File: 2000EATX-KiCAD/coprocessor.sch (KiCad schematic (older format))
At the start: 31 parts, among them CN600 Amiga-2000-CPU-Slot, U600 74LS245, U601 74LS245, U602 74LS245, U603 74LS245, U604 74LS245, U605 74LS245

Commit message: Add files via upload
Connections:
- wire segments 343 -> 338
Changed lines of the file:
@@
 $Descr A4 11693 8268
 encoding utf-8
-Sheet 4 9
+Sheet 4 10
 Title ""
 Date ""
@@
 	1500 1550 1500 1600
 $Comp
-L Amiga~3000~library:GND #PWR0123
+L power:GND #PWR0123
 U 1 1 604D2A89
 P 1500 6250
@@
 Connection ~ 2100 1750
 $Comp
-L Amiga~3000~library:+5V #PWR0124
+L power:+5V #PWR0124
 U 1 1 604D882A
 P 2100 1550
@@
 $EndComp
 $Comp
-L Amiga~3000~library:-5V #PWR0125
+L power:-5V #PWR0125
 U 1 1 604D8A9E
 P 2250 1350
@@
 $EndComp
 $Comp
-L Amiga~3000~library:+12V #PWR0126
+L power:+12V #PWR0126
 U 1 1 604DB1C1
 P 2400 1550
@@
 NoConn ~ 5300 1800
 $Comp
-L Amiga~3000~library:GND #PWR0127
+L power:GND #PWR0127
 U 1 1 60551069
 P 5800 2400
@@
 $EndComp
 $Comp
-L Amiga~3000~library:GND #PWR0128
+L power:GND #PWR0128
 U 1 1 6056F1B9
 P 6850 4150
@@
 $EndComp
 $Comp
-L Amiga~3000~library:GND #PWR0129
+L power:GND #PWR0129
 U 1 1 6056F9E8
 P 5850 5650
@@
 BD8
 $Comp
-L Amiga~3000~library:GND #PWR0130
+L power:GND #PWR0130
 U 1 1 605B732B
 P 10250 2800
@@
 $EndComp
 $Comp
-L Amiga~3000~library:GND #PWR0131
+L power:GND #PWR0131
 U 1 1 605B78D1
 P 10250 5050
@@
 	9750 4450 8800 4450
 $Comp
-L Amiga~3000~library:GND #PWR0132
+L power:GND #PWR0132
 U 1 1 607375B5
 P 7850 1800
@@
 $EndComp
 $Comp
-L Amiga~3000~library:GND #PWR0133
+L power:GND #PWR0133
 U 1 1 6073AFFD
 P 7900 4250
@@
 _BAS
 $Comp
-L Amiga~3000~library:GND #PWR0134
+L power:GND #PWR0134
 U 1 1 60B411F4
 P 3750 7500
@@
 $EndComp
 $Comp
-L Amiga~3000~library:+5V #PWR0135
+L power:+5V #PWR0135
 U 1 1 60B454E3
 P 4400 5650
 F 0 "#PWR0135" H 4400 5500 50  0001 C CNN
-F 1 "+5V" H 4417 5873 50  0000 C CNN
+F 1 "+5V" H 4400 5800 50  0000 C CNN
 F 2 "" H 4400 5650 50  0001 C CNN
 F 3 "" H 4400 5650 50  0001 C CNN
@@
 $EndComp
 $Comp
-L Amiga~3000~library:GND #PWR0136
+L power:GND #PWR0136
 U 1 1 60B78755
 P 3250 7200
@@
 $EndComp
 $Comp
-L Amiga~3000~library:+5V #PWR0137
+L power:+5V #PWR0137
 U 1 1 60E422B1
 P 3450 5800
@@
 $EndComp
 $Comp
-L Amiga~3000~library:GND #PWR0138
+L power:GND #PWR0138
 U 1 1 60E42986
 P 3150 5800
@@
 Wire Wire Line
 	3450 5900 3750 5900
-Connection ~ 3450 5800
 $Comp
 L Device:C_Small C602
@@
 $EndComp
 $Comp
-L Amiga~3000~library:GND #PWR0139
+L power:GND #PWR0139
 U 1 1 60E7B497
 P 10900 3450
@@
 $EndComp
 $Comp
-L Amiga~3000~library:GND #PWR0140
+L power:GND #PWR0140
 U 1 1 60E7BCF4
 P 10800 1200
@@
 $EndComp
 $Comp
-L Amiga~3000~library:GND #PWR0141
+L power:GND #PWR0141
 U 1 1 60E7CCB0
 P 6350 800
@@
 $EndComp
 $Comp
-L Amiga~3000~library:GND #PWR0142
+L power:GND #PWR0142
 U 1 1 60E7E9FD
 P 7500 2400
@@
 $EndComp
 $Comp
-L Amiga~3000~library:+5V #PWR0143
+L power:+5V #PWR0143
 U 1 1 60E89AA3
 P 6150 4150
@@
 	4200 850  4200 3750
 $Comp
-L Amiga~3000~library:+5V #PWR0144
+L power:+5V #PWR0144
 U 1 1 60FCDD63
 P 7150 2400
@@
 	1    0    0    -1
 $EndComp
-Wire Wire Line
-	7300 2400 7150 2400
-Connection ~ 7150 2400
-Wire Wire Line
-	7150 2400 6850 2400
-$Comp
-L Amiga~3000~library:+5V #PWR0145
+$Comp
+L power:+5V #PWR0145
 U 1 1 60FE91B2
 P 6050 800
@@
 $EndComp
 $Comp
-L Amiga~3000~library:+5V #PWR0146
+L power:+5V #PWR0146
 U 1 1 60FE967D
 P 10500 1200
@@
 $EndComp
 $Comp
-L Amiga~3000~library:+5V #PWR0147
+L power:+5V #PWR0147
 U 1 1 60FE9CDB
 P 10500 3450
@@
 	1    0    0    -1
 $EndComp
-Wire Wire Line
-	10250 3450 10500 3450
-Connection ~ 10500 3450
-Wire Wire Line
-	10500 3450 10700 3450
-Wire Wire Line
-	10600 1200 10500 1200
-Connection ~ 10500 1200
-Wire Wire Line
-	10500 1200 10250 1200
-Wire Wire Line
-	5800 800  6050 800
-Connection ~ 6050 800
-Wire Wire Line
-	6050 800  6150 800
-$Comp
-L Amiga~3000~library:GND #PWR0148
+$Comp
+L power:GND #PWR0148
 U 1 1 610452A3
 P 5300 2100
@@
 $EndComp
 $Comp
-L Amiga~3000~library:GND #PWR0149
+L power:GND #PWR0149
 U 1 1 61045A56
 P 5350 5350
@@
 $EndComp
 $Comp
-L Amiga~3000~library:GND #PWR0150
+L power:GND #PWR0150
 U 1 1 610463ED
 P 6350 3700
@@
 Wire Wire Line
 	6850 4150 6850 4000
-Connection ~ 6850 4150
-Wire Wire Line
-	6500 4150 6150 4150
 Wire Wire Line
 	5850 4050 6000 4050
 Wire Wire Line
 	6000 4050 6000 4150
-Wire Wire Line
-	6000 4150 6150 4150
-Connection ~ 6150 4150
 Text GLabel 7450 4950 0    47   Input ~ 0
 _DBOE
@@
 Wire Wire Line
 	3100 1700 3100 2550
+Wire Wire Line
+	6850 2400 7300 2400
+Wire Wire Line
+	10250 3450 10700 3450
+Wire Wire Line
+	10250 1200 10600 1200
+Wire Wire Line
+	5800 800  6150 800
+Wire Wire Line
+	6000 4150 6500 4150
 $EndSCHEMATC

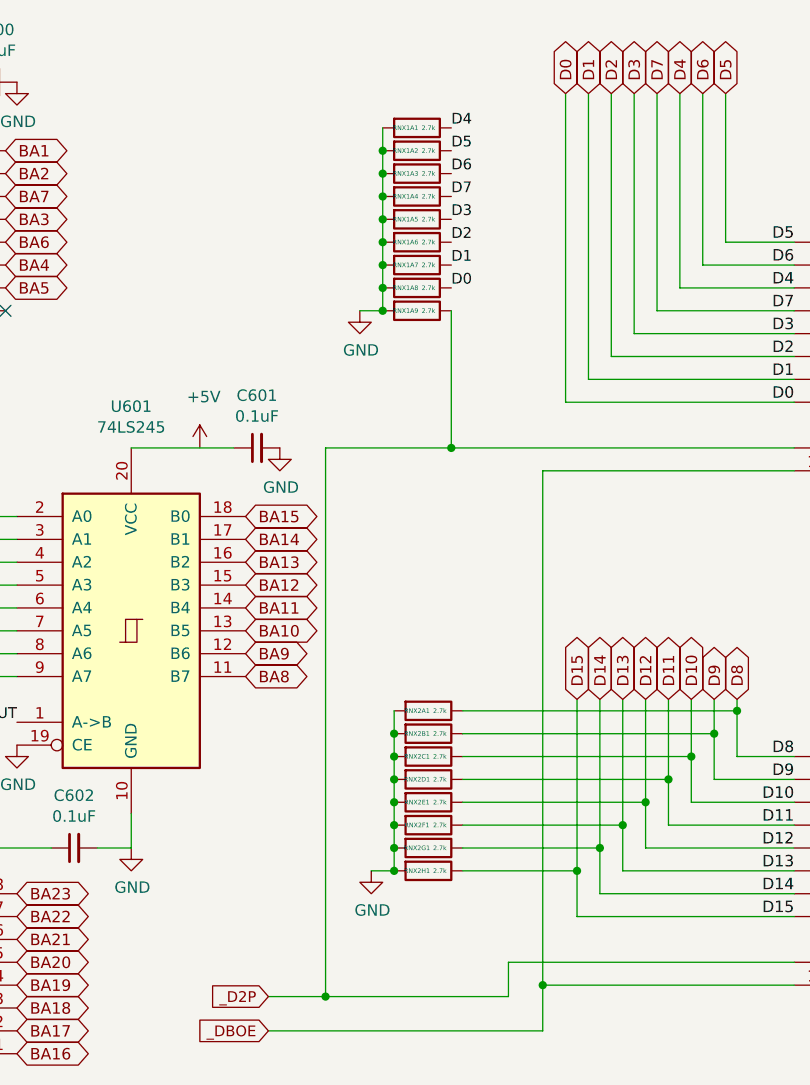
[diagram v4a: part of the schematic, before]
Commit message: Add files via upload
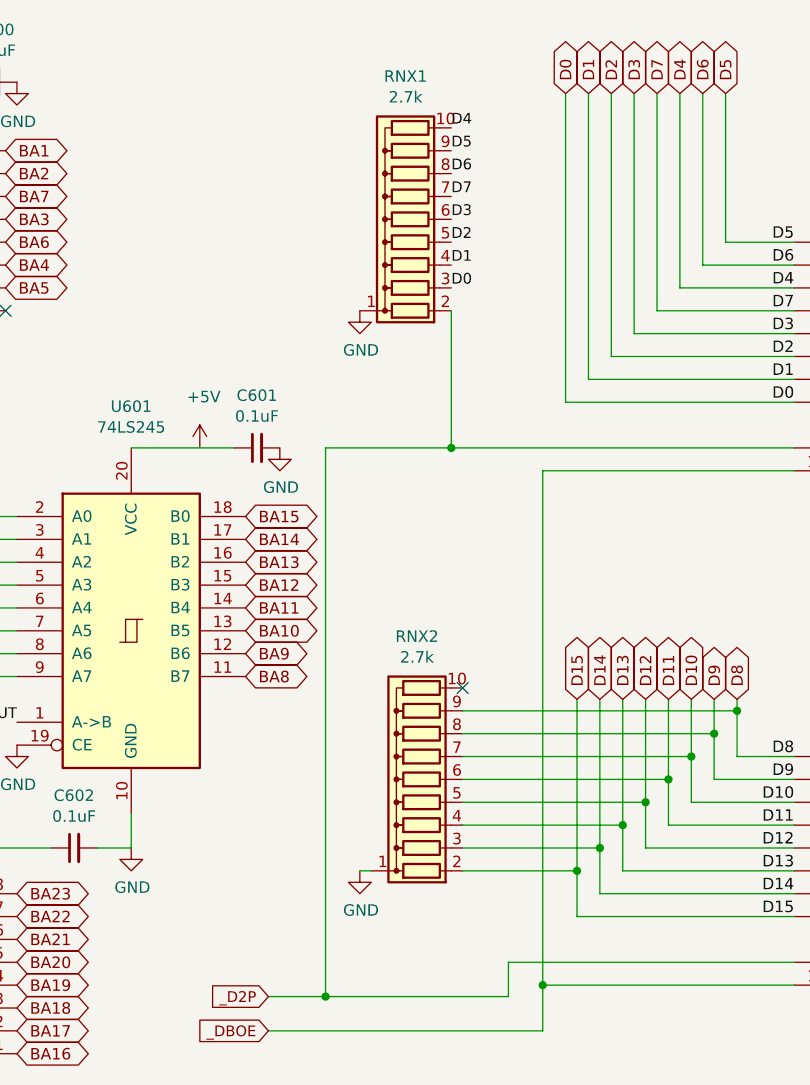
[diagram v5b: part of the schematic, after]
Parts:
- removed RNX1A1, RNX1A2, RNX1A3, RNX1A4, RNX1A5, RNX1A6, RNX1A7, RNX1A8, RNX1A9, RNX2A1, RNX2B1, RNX2C1, RNX2D1, RNX2E1, RNX2F1, RNX2G1, RNX2H1: 2.7k, Resistor_SMD:R_1206_3216Metric, symbol Device:R
- added RNX1, RNX2: 2.7k, Resistor_THT:R_Array_SIP10, symbol Device:R_Network09
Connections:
- net D0: now also RNX1.3 (R2)
- net D1: now also RNX1.4 (R3)
- net D10: now also RNX2.7 (R6)
- net D11: now also RNX2.6 (R5)
- net D12: now also RNX2.5 (R4)
- net D13: now also RNX2.4 (R3)
- net D14: now also RNX2.3 (R2)
- net D15: now also RNX2.2 (R1)
- net D2: now also RNX1.5 (R4)
- net D3: now also RNX1.6 (R5)
- net D4: now also RNX1.10 (R9)
- net D5: now also RNX1.9 (R8)
- net D6: now also RNX1.8 (R7)
- net D7: now also RNX1.7 (R6)
- net D8: now also RNX2.9 (R8)
- net D9: now also RNX2.8 (R7)
- net GND: now also RNX1.1 (common), RNX2.1 (common)
- net _D2P: now also RNX1.2 (R1)
- no-connect marks 2 -> 3

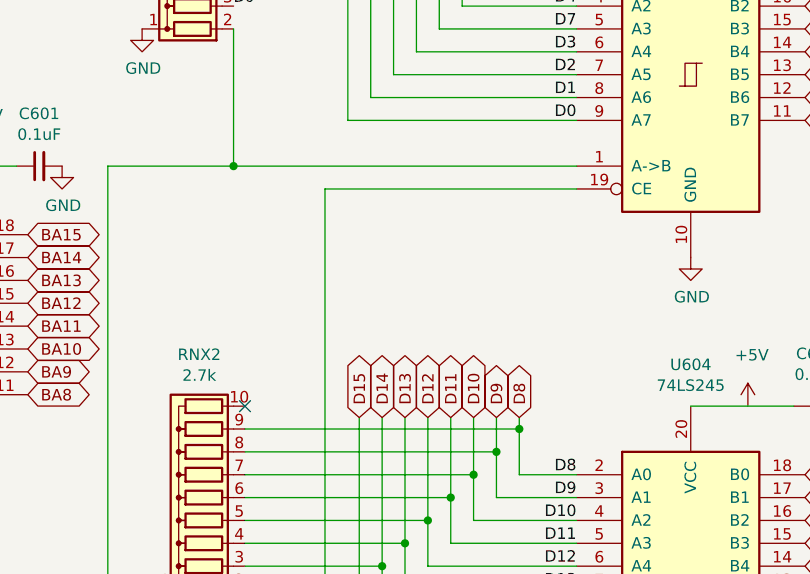
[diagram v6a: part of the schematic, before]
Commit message: Add files via upload
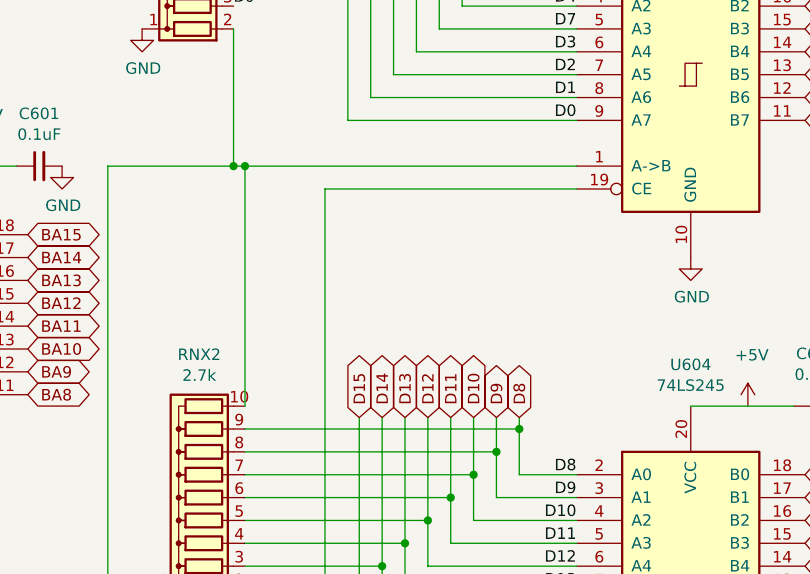
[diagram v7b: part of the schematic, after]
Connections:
- net _D2P: now also RNX2.10 (R9)
- no-connect marks 3 -> 2
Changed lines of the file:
@@
 Connection ~ 8250 2400
 Wire Wire Line
-	8250 2400 9750 2400
+	8250 2400 8300 2400
 Wire Wire Line
 	7450 4950 8650 4950
@@
 Wire Wire Line
 	7850 4250 7900 4250
-NoConn ~ 8300 3450
+Wire Wire Line
+	8300 3450 8300 2400
+Connection ~ 8300 2400
+Wire Wire Line
+	8300 2400 9750 2400
 $EndSCHEMATC

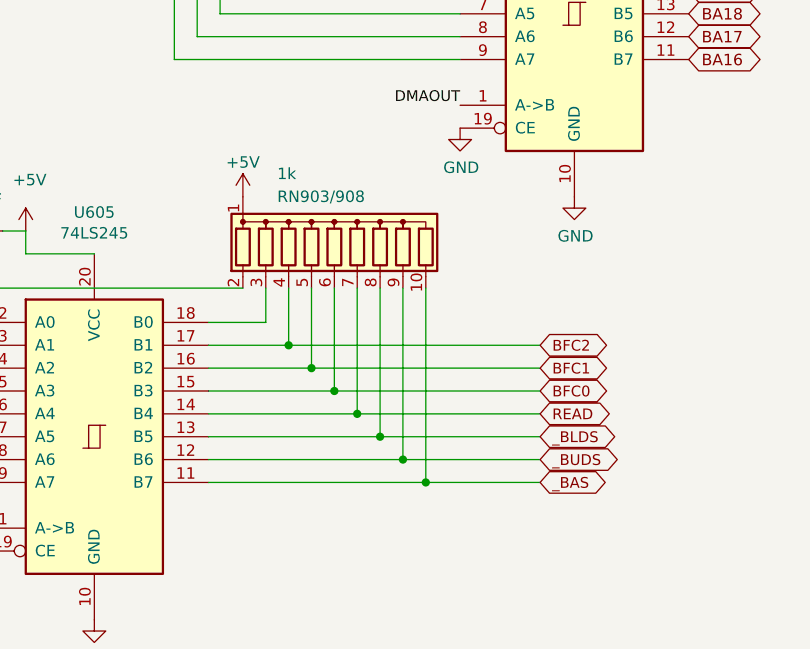
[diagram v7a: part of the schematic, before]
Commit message: Add files via upload
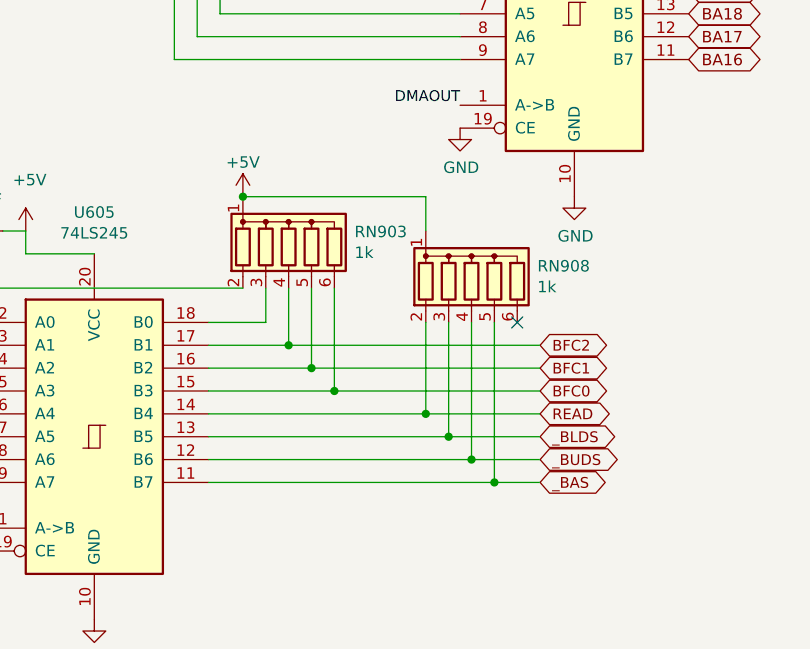
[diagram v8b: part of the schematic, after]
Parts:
- removed RN903/908: 1k, Resistor_THT:R_Array_SIP11, symbol Device:R_Network09
- added RN903, RN908: 1k, Resistor_THT:R_Array_SIP6, symbol Device:R_Network05
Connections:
- net +5V: now also RN903.1 (common), RN908.1 (common)
- net BFC0: now also RN903.6 (R5)
- net BFC1: now also RN903.5 (R4)
- net BFC2: now also RN903.4 (R3)
- net READ: now also RN908.2 (R1)
- net _BAS: now also RN908.5 (R4)
- net _BLDS: now also RN908.3 (R2)
- net _BUDS: now also RN908.4 (R3)
- net at U605.18 (B0): now also RN903.3 (R2)
- net at U605.2 (A0): now also RN903.2 (R1)
- no-connect marks 2 -> 3
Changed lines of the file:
@@
-$EndComp
-$Comp
-L Device:R_Network09 RN903/908
-U 1 1 60B42275
-P 4800 5850
-F 0 "RN903/908" H 4550 6050 50  0000 L CNN
-F 1 "1k" H 4550 6150 50  0000 L CNN
-F 2 "Resistor_THT:R_Array_SIP11" V 5375 5850 50  0001 C CNN
-F 3 "http://www.vishay.com/docs/31509/csc.pdf" H 4800 5850 50  0001 C CNN
-	1    4800 5850
-	1    0    0    -1
 $EndComp
 $Comp
@@
 Wire Wire Line
 	4250 6500 4800 6500
-Wire Wire Line
-	4250 6600 4900 6600
-Wire Wire Line
-	4250 6700 5000 6700
-Wire Wire Line
-	4250 6800 5100 6800
-Wire Wire Line
-	5200 6050 5200 6900
-Wire Wire Line
-	4250 6900 5200 6900
-Connection ~ 5200 6900
-Wire Wire Line
-	5200 6900 5700 6900
-Wire Wire Line
-	5100 6050 5100 6800
-Connection ~ 5100 6800
-Wire Wire Line
-	5100 6800 5700 6800
-Wire Wire Line
-	5000 6050 5000 6700
-Connection ~ 5000 6700
-Wire Wire Line
-	5000 6700 5700 6700
-Wire Wire Line
-	4900 6050 4900 6600
-Connection ~ 4900 6600
-Wire Wire Line
-	4900 6600 5700 6600
 Wire Wire Line
 	4800 6050 4800 6500
@@
 Wire Wire Line
 	8300 2400 9750 2400
+$Comp
+L Device:R_Network05 RN903
+U 1 1 61444A0D
+P 4600 5850
+F 0 "RN903" H 4888 5896 50  0000 L CNN
+F 1 "1k" H 4888 5805 50  0000 L CNN
+F 2 "Resistor_THT:R_Array_SIP6" V 4975 5850 50  0001 C CNN
+F 3 "http://www.vishay.com/docs/31509/csc.pdf" H 4600 5850 50  0001 C CNN
+	1    4600 5850
+	1    0    0    -1
+$EndComp
+$Comp
+L Device:R_Network05 RN908
+U 1 1 61446021
+P 5400 6000
+F 0 "RN908" H 5688 6046 50  0000 L CNN
+F 1 "1k" H 5688 5955 50  0000 L CNN
+F 2 "Resistor_THT:R_Array_SIP6" V 5775 6000 50  0001 C CNN
+F 3 "http://www.vishay.com/docs/31509/csc.pdf" H 5400 6000 50  0001 C CNN
+	1    5400 6000
+	1    0    0    -1
+$EndComp
+Wire Wire Line
+	4250 6600 5200 6600
+Wire Wire Line
+	4250 6700 5300 6700
+Wire Wire Line
+	4250 6800 5400 6800
+Wire Wire Line
+	4250 6900 5500 6900
+Wire Wire Line
+	5200 5800 5200 5650
+Wire Wire Line
+	5200 5650 4400 5650
+Connection ~ 4400 5650
+Wire Wire Line
+	5200 6200 5200 6600
+Connection ~ 5200 6600
+Wire Wire Line
+	5200 6600 5700 6600
+Wire Wire Line
+	5300 6200 5300 6700
+Connection ~ 5300 6700
+Wire Wire Line
+	5300 6700 5700 6700
+Wire Wire Line
+	5400 6200 5400 6800
+Connection ~ 5400 6800
+Wire Wire Line
+	5400 6800 5700 6800
+Wire Wire Line
+	5500 6200 5500 6900
+Connection ~ 5500 6900
+Wire Wire Line
+	5500 6900 5700 6900
+NoConn ~ 5600 6200
 $EndSCHEMATC
